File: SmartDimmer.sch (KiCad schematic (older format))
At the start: 86 parts, among them J1 Conn_01x02, J10 Conn_01x05, J11 Conn_01x02, J12 Conn_01x02, J13 Conn_01x02, J14 Conn_01x02, J2 Conn_01x04, J3 Conn_01x02, J4 Conn_01x08, J5 Conn_01x04, J6 Conn_01x02, J8 Conn_01x02, J9 Conn_01x02, Q1 2N7000, Q2 2N7000, Q3 2N7000, Q4 2N7000, Q5 Q_NPN_EBC, Q6 Q_NPN_EBC, SW1 SW_Push, T1 TouchPad, T2 TouchPad, U1 ESP32-WROOM, U10 ACS712, U11 ACS712, U2 AT42QT1010-TSHR, U3 FL5160, U4 FL5160, U5 IPD50R399CP, U6 IPD50R399CP, U7 IPD50R399CP, U8 IPD50R399CP, U9 AT42QT1010-TSHR

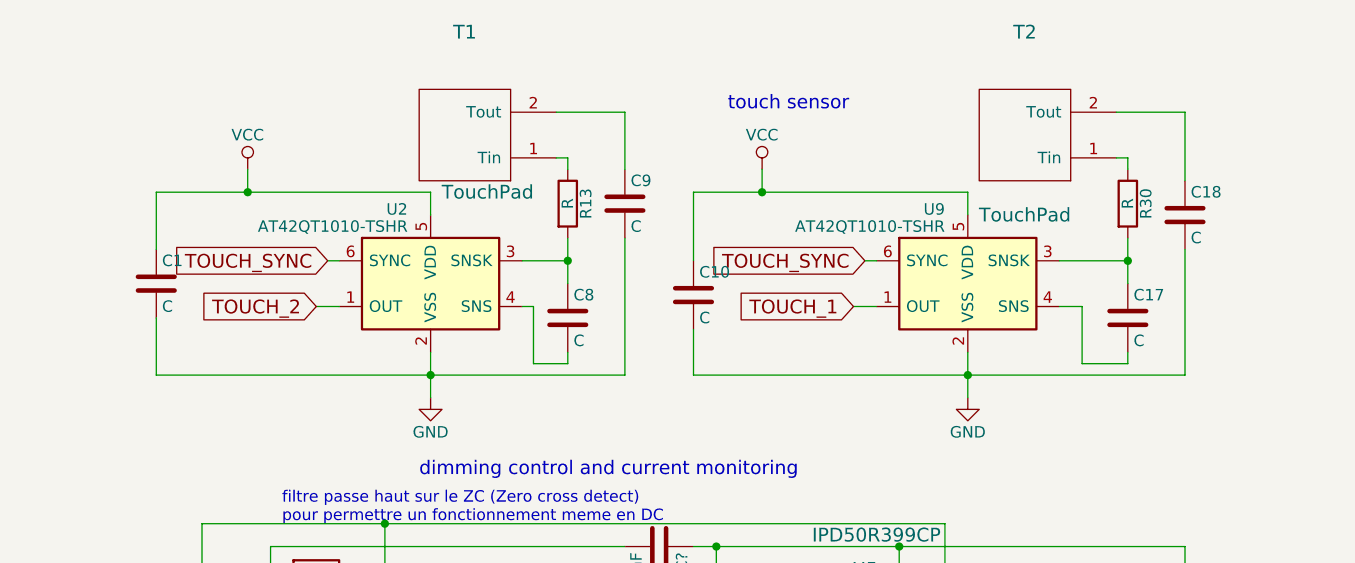
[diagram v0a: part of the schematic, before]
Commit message: added datasheet
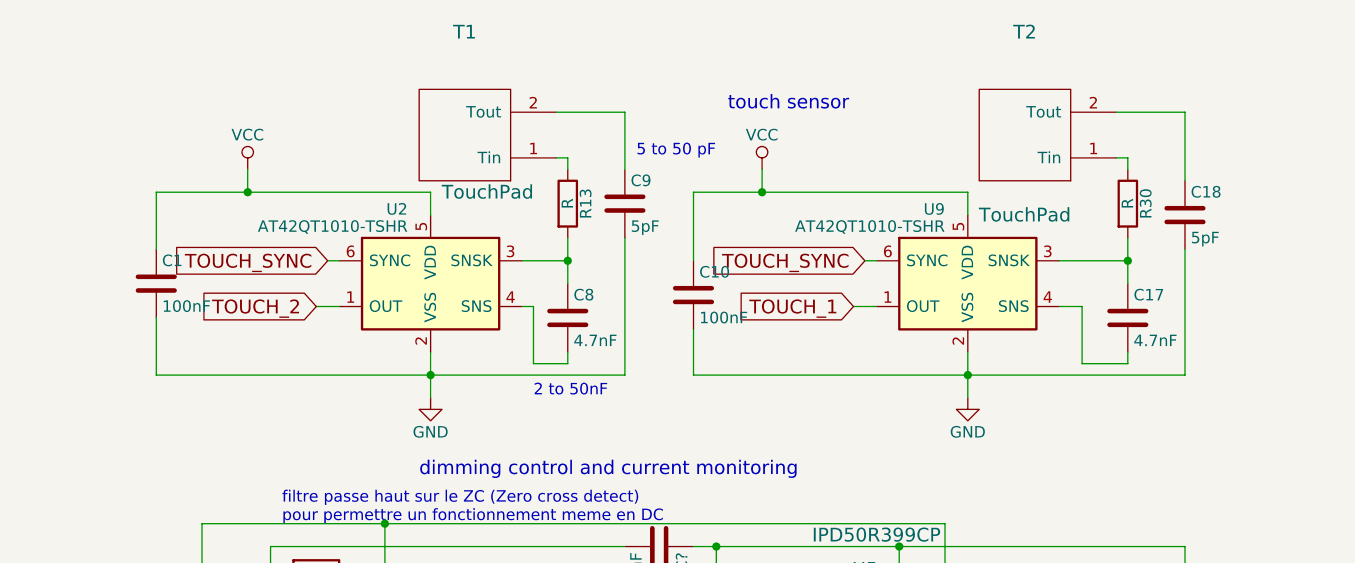
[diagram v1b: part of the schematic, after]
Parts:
- C1, C10: value C -> 100nF
- C17, C8: value C -> 4.7nF
- C18, C9: value C -> 5pF
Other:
- note added: "2 to 50nF"
- note added: "5 to 50 pF"
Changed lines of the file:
@@
 P 6150 1400
 F 0 "C1" H 6175 1500 50  0000 L CNN
-F 1 "C" H 6175 1300 50  0000 L CNN
+F 1 "100nF" H 6175 1300 50  0000 L CNN
 F 2 "" H 6188 1250 50  0001 C CNN
 F 3 "" H 6150 1400 50  0001 C CNN
@@
 P 8500 1450
 F 0 "C10" H 8525 1550 50  0000 L CNN
-F 1 "C" H 8525 1350 50  0000 L CNN
+F 1 "100nF" H 8525 1350 50  0000 L CNN
 F 2 "" H 8538 1300 50  0001 C CNN
 F 3 "" H 8500 1450 50  0001 C CNN
@@
 P 10400 1550
 F 0 "C17" H 10425 1650 50  0000 L CNN
-F 1 "C" H 10425 1450 50  0000 L CNN
+F 1 "4.7nF" H 10425 1450 50  0000 L CNN
 F 2 "" H 10438 1400 50  0001 C CNN
 F 3 "" H 10400 1550 50  0001 C CNN
@@
 P 7950 1550
 F 0 "C8" H 7975 1650 50  0000 L CNN
-F 1 "C" H 7975 1450 50  0000 L CNN
+F 1 "4.7nF" H 7975 1450 50  0000 L CNN
 F 2 "" H 7988 1400 50  0001 C CNN
 F 3 "" H 7950 1550 50  0001 C CNN
@@
 P 10650 1100
 F 0 "C18" H 10675 1200 50  0000 L CNN
-F 1 "C" H 10675 1000 50  0000 L CNN
+F 1 "5pF" H 10675 1000 50  0000 L CNN
 F 2 "" H 10688 950 50  0001 C CNN
 F 3 "" H 10650 1100 50  0001 C CNN
@@
 P 8200 1050
 F 0 "C9" H 8225 1150 50  0000 L CNN
-F 1 "C" H 8225 950 50  0000 L CNN
+F 1 "5pF" H 8225 950 50  0000 L CNN
 F 2 "" H 8238 900 50  0001 C CNN
 F 3 "" H 8200 1050 50  0001 C CNN
@@
 Text Notes 7150 4900 0    50   ~ 0
 (condo >300V V)
+Text Notes 7800 1900 0    50   ~ 0
+2 to 50nF
+Text Notes 8250 850  0    50   ~ 0
+5 to 50 pF
 $EndSCHEMATC

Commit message: Rework of the schematic and started the layout
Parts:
- removed J2: Conn_01x04, symbol SmartDimmer-rescue:Conn_01x04
- removed J4: Conn_01x08, symbol SmartDimmer-rescue:Conn_01x08
- removed Q3, Q4: 2N7000, TO_SOT_Packages_THT:TO-92_Molded_Narrow, symbol SmartDimmer-rescue:2N7000
- removed R11, R12, R7, R8: 10k, symbol Device:R
- removed R26, R27, R28, R29: R, symbol Device:R
- removed T1, T2: TouchPad, symbol DimmerComponent:TouchPad
- added C?: 100nF, symbol Device:C
- added C?: 3uF, symbol Device:C
- added J7, J9: Conn_01x08, Connector_PinHeader_2.54mm:PinHeader_1x08_P2.54mm_Vertical, symbol Connector_Generic:Conn_01x08
- added R? (x2): 10K, symbol Device:R
- added R? (x2): 100R, symbol Device:R
- added T1, T2: Conn_01x01, Connector_PinHeader_2.54mm:PinHeader_1x01_P2.54mm_Vertical, symbol Connector_Generic:Conn_01x01
- added U? (x6): TCMT1100, Package_SO:SOP-4_4.4x2.8mm_P1.27mm, symbol Isolator:TCMT1100
- C1: footprint (none) -> Capacitor_SMD:C_1206_3216Metric_Pad1.42x1.75mm_HandSolder
- C10: renamed from C5; footprint (none) -> Capacitor_SMD:C_1206_3216Metric_Pad1.42x1.75mm_HandSolder
- C11: renamed from C6; value 1uF -> 3uF; footprint (none) -> Capacitor_SMD:C_1206_3216Metric_Pad1.42x1.75mm_HandSolder
- C12: renamed from C7; value 1uF -> 3uF; footprint (none) -> Capacitor_SMD:C_1206_3216Metric_Pad1.42x1.75mm_HandSolder
- C13, C14: renamed from C?; footprint (none) -> Capacitor_SMD:C_1206_3216Metric_Pad1.42x1.75mm_HandSolder
- C15: renamed from C11; footprint (none) -> Capacitor_SMD:C_1206_3216Metric_Pad1.42x1.75mm_HandSolder
- C16: renamed from C12; footprint (none) -> Capacitor_SMD:C_1206_3216Metric_Pad1.42x1.75mm_HandSolder
- C17: renamed from C13; footprint (none) -> Capacitor_SMD:C_1206_3216Metric_Pad1.42x1.75mm_HandSolder
- C18: renamed from C14; footprint (none) -> Capacitor_SMD:C_1206_3216Metric_Pad1.42x1.75mm_HandSolder
- C19: renamed from C15; footprint (none) -> Capacitor_SMD:C_1206_3216Metric_Pad1.42x1.75mm_HandSolder
- C2: renamed from C8; footprint (none) -> Capacitor_SMD:C_1206_3216Metric_Pad1.42x1.75mm_HandSolder
- C20: renamed from C16; footprint (none) -> Capacitor_SMD:C_1206_3216Metric_Pad1.42x1.75mm_HandSolder
- C3: renamed from C9; footprint (none) -> Capacitor_SMD:C_1206_3216Metric_Pad1.42x1.75mm_HandSolder
- C4: renamed from C10; footprint (none) -> Capacitor_SMD:C_1206_3216Metric_Pad1.42x1.75mm_HandSolder
- C5: renamed from C17; footprint (none) -> Capacitor_SMD:C_1206_3216Metric_Pad1.42x1.75mm_HandSolder
- C6: renamed from C18; footprint (none) -> Capacitor_SMD:C_1206_3216Metric_Pad1.42x1.75mm_HandSolder
- C7: renamed from C2; footprint (none) -> Capacitor_SMD:C_1206_3216Metric_Pad1.42x1.75mm_HandSolder
- C8: renamed from C3; footprint (none) -> Capacitor_SMD:C_1206_3216Metric_Pad1.42x1.75mm_HandSolder
- C9: renamed from C4; footprint (none) -> Capacitor_SMD:C_1206_3216Metric_Pad1.42x1.75mm_HandSolder
- D1: footprint (none) -> LED_SMD:LED_1206_3216Metric_Pad1.42x1.75mm_HandSolder
- D2: renamed from D3; footprint (none) -> Diode_SMD:D_1206_3216Metric_Pad1.42x1.75mm_HandSolder
- D3: renamed from D2; footprint (none) -> Diode_SMD:D_1206_3216Metric_Pad1.42x1.75mm_HandSolder
- J1, J8: footprint (none) -> Connector_PinHeader_2.54mm:PinHeader_1x02_P2.54mm_Vertical
- J10: renamed from J11; footprint (none) -> Connector_PinHeader_2.54mm:PinHeader_1x02_P2.54mm_Vertical
- J11: renamed from J12; footprint (none) -> TerminalBlock_RND:TerminalBlock_RND_205-00012_1x02_P5.00mm_Horizontal
- J12: renamed from J13; footprint (none) -> TerminalBlock_RND:TerminalBlock_RND_205-00012_1x02_P5.00mm_Horizontal
- J13: renamed from J14; footprint (none) -> TerminalBlock_RND:TerminalBlock_RND_205-00012_1x02_P5.00mm_Horizontal
- J2: renamed from J3; footprint (none) -> Connector_PinHeader_2.54mm:PinHeader_1x02_P2.54mm_Vertical
- J3: renamed from J5; footprint (none) -> Connector_PinHeader_2.54mm:PinHeader_1x04_P2.54mm_Vertical
- J4: renamed from J6; footprint (none) -> Connector_PinHeader_2.54mm:PinHeader_1x02_P2.54mm_Vertical
- J5: renamed from J9; footprint (none) -> Connector_PinHeader_2.54mm:PinHeader_1x02_P2.54mm_Vertical
- J6: renamed from J10; footprint (none) -> Connector_PinHeader_2.54mm:PinHeader_1x05_P2.54mm_Vertical
- Q1, Q2: footprint TO_SOT_Packages_THT:TO-92_Molded_Narrow -> Package_TO_SOT_SMD:SOT-23_Handsoldering
- Q5, Q6: footprint (none) -> Package_TO_SOT_SMD:SOT-23_Handsoldering
- R1, R2, R3, R4: footprint (none) -> Resistor_SMD:R_1206_3216Metric_Pad1.42x1.75mm_HandSolder
- R11: renamed from R9; footprint (none) -> Resistor_SMD:R_1206_3216Metric_Pad1.42x1.75mm_HandSolder
- R12: renamed from R10; footprint (none) -> Resistor_SMD:R_1206_3216Metric_Pad1.42x1.75mm_HandSolder
- R15, R16: renamed from R?; footprint (none) -> Resistor_SMD:R_1206_3216Metric_Pad1.42x1.75mm_HandSolder
- R17: renamed from R15; footprint (none) -> Resistor_SMD:R_1206_3216Metric_Pad1.42x1.75mm_HandSolder
- R18: renamed from R16; footprint (none) -> Resistor_SMD:R_1206_3216Metric_Pad1.42x1.75mm_HandSolder
- R19: renamed from R17; footprint (none) -> Resistor_SMD:R_1206_3216Metric_Pad1.42x1.75mm_HandSolder
- R20: renamed from R19; footprint (none) -> Resistor_SMD:R_1206_3216Metric_Pad1.42x1.75mm_HandSolder
- R21: renamed from R20; footprint (none) -> Resistor_SMD:R_1206_3216Metric_Pad1.42x1.75mm_HandSolder
- R22: renamed from R21; footprint (none) -> Resistor_SMD:R_1206_3216Metric_Pad1.42x1.75mm_HandSolder
- R23: renamed from R22; footprint (none) -> Resistor_SMD:R_1206_3216Metric_Pad1.42x1.75mm_HandSolder
- R24: renamed from R23; footprint (none) -> Resistor_SMD:R_1206_3216Metric_Pad1.42x1.75mm_HandSolder
- R25: renamed from R24; footprint (none) -> Resistor_SMD:R_1206_3216Metric_Pad1.42x1.75mm_HandSolder
- R26: renamed from R25; footprint (none) -> Resistor_SMD:R_1206_3216Metric_Pad1.42x1.75mm_HandSolder
- R5: renamed from R13; value R -> 100K; footprint (none) -> Resistor_SMD:R_1206_3216Metric_Pad1.42x1.75mm_HandSolder
- R6: renamed from R5; footprint (none) -> Resistor_SMD:R_1206_3216Metric_Pad1.42x1.75mm_HandSolder
- R7: renamed from R6; footprint (none) -> Resistor_SMD:R_1206_3216Metric_Pad1.42x1.75mm_HandSolder
- R8: renamed from R30; value R -> 100K; footprint (none) -> Resistor_SMD:R_1206_3216Metric_Pad1.42x1.75mm_HandSolder
- SW1: footprint (none) -> Button_Switch_SMD:SW_SPST_FSMSM
- U1: renamed from U2; footprint TO_SOT_Packages_SMD:SOT-23-6 -> Package_TO_SOT_SMD:SOT-23-6
- U10, U11: footprint (none) -> Package_SO:SOIC-8_3.9x4.9mm_P1.27mm
- U3: renamed from U9; footprint TO_SOT_Packages_SMD:SOT-23-6 -> Package_TO_SOT_SMD:SOT-23-6
- U4: renamed from U3; footprint (none) -> Package_SO:SSOP-10_3.9x4.9mm_P1.00mm
- U5: renamed from U4; footprint (none) -> Package_SO:SSOP-10_3.9x4.9mm_P1.00mm
- U6: renamed from U5; footprint (none) -> Package_TO_SOT_SMD:TO-252-2
- U7: renamed from U6; footprint (none) -> Package_TO_SOT_SMD:TO-252-2
- U8: renamed from U7; footprint (none) -> Package_TO_SOT_SMD:TO-252-2
- U9: renamed from U8; footprint (none) -> Package_TO_SOT_SMD:TO-252-2
- renumbered U1 to U2
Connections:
- net VDD is gone; now on net VCC: J6.2 (Pin_2)
- net Current_Meas_1: now also J7.4 (Pin_4)
- net Current_Meas_2: now also J7.7 (Pin_7)
- net DIM_Control_1: no longer R11.2
- net DIM_Control_2: now also J7.5 (Pin_5); no longer R12.2
- net DIM_MODE_1: now also U?.1
- net DIM_MODE_2: now also U?.1
- net GND: now also C?.2, C?.2, R?.2, R?.2; no longer C10.1, C11.2, C12.2, C17.1, C18.1, C19.2, C20.2, C7.2, C8.1, C9.2, U10.5 (GND), U11.5 (GND), U4.5 (GND), U5.5 (GND)
- net VCC: now also C?.1, C?.1
- net at U5.4 (DIM_Mode): now also J9.6 (Pin_6)
- net HV_9: now reaches Q6.2 (B), R25.2, U5.7 (Low_Power)
- net PWR_1: now reaches C13.1, J13.1 (Pin_1), R20.1, U8.2
- net PWR_1: no longer U11.1 (IP+), U11.2 (IP+)
- net PWR_2: now reaches R22.1, U11.3 (IP-), U11.4 (IP-), U9.2
- net PWR_2: no longer J13.2 (Pin_2)
- net at U11.7 (VIOUT): now also J9.7 (Pin_7)
- net HV_2: now reaches D3.2 (A), J10.1 (Pin_1), J11.1 (Pin_1)
- net HV_3: now reaches D2.2 (A), J10.2 (Pin_2), J11.2 (Pin_2)
- net GND_PWR: now reaches C16.1, U8.3, U9.3
- net GND_PWR: now also C10.1, C15.1, C17.1, C18.1, C19.2, C20.2, C7.2, C8.1, C9.2, U10.5 (GND), U11.5 (GND), U4.5 (GND), U5.5 (GND), U6.3, U7.3, J9.8 (Pin_8)
- net HV_5: now reaches Q6.3 (C), R26.2
- net at R8.1: now also C6.1, T1.1 (Pin_1)
- net at R5.1: now also C3.1, T2.1 (Pin_1)
- net at U4.4 (DIM_Mode): now also J9.3 (Pin_3)
- net HV_6: now reaches Q5.2 (B), R23.2, U4.7 (Low_Power)
- net PWR_6: now reaches C14.1, J12.1 (Pin_1), R17.1, U6.2
- net PWR_6: no longer U10.1 (IP+), U10.2 (IP+)
- net PWR_4: now reaches R19.1, U10.3 (IP-), U10.4 (IP-), U7.2
- net PWR_4: no longer J12.2 (Pin_2)
- net at U10.7 (VIOUT): now also J9.4 (Pin_4)
- net HV_8: now reaches Q5.3 (C), R24.2
- new net: J9.5 (Pin_5), U5.2 (DIM_Control)
- new net: J9.2 (Pin_2), U4.2 (DIM_Control)
- new net: J7.1 (Pin_1), U?.4, U?.4
- new net: J7.2 (Pin_2), U?.4
- new net: J7.3 (Pin_3), R?.1, U?.3
- new net: J7.6 (Pin_6), R?.1, U?.3
- new net: J7.8 (Pin_8), R?.2, R?.2, U?.3
- new net: R?.1, U?.2 (x2)
- new net PWR_3: J13.2 (Pin_2), U11.1 (IP+), U11.2 (IP+)
- new net PWR_5: J12.2 (Pin_2), U10.1 (IP+), U10.2 (IP+)
- new net VCC_PWR: J9.1 (Pin_1)
- now unconnected: C11.1, C12.1, R11.1, R12.1
- no-connect marks 1 -> 13
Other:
- note added: "ADC voltage\nreference : 2.5V"
- note added: "Add galvanic isolation (Optocoupler)\n"
- note added: "BOARD 230VAC"
- note added: "BOARD DC\n"
- note added: "VDD provide 5V for the ACS712"
- note added: "Voltage Divider 5V to 3V3,\nResistor real ration < 0.66"
- note removed: "Dimmensionnement :\n"
- moved on the sheet: C1, C10, C11, C12, C13, C14, C15, C16, C17, C18, C19, C2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
